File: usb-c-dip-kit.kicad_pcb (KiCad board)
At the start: 2 copper layers, 13.8 x 18.3 mm, 4 parts, among them CN1 USB2.0_C_12pin, CN2 USB_C_DIP_Socket

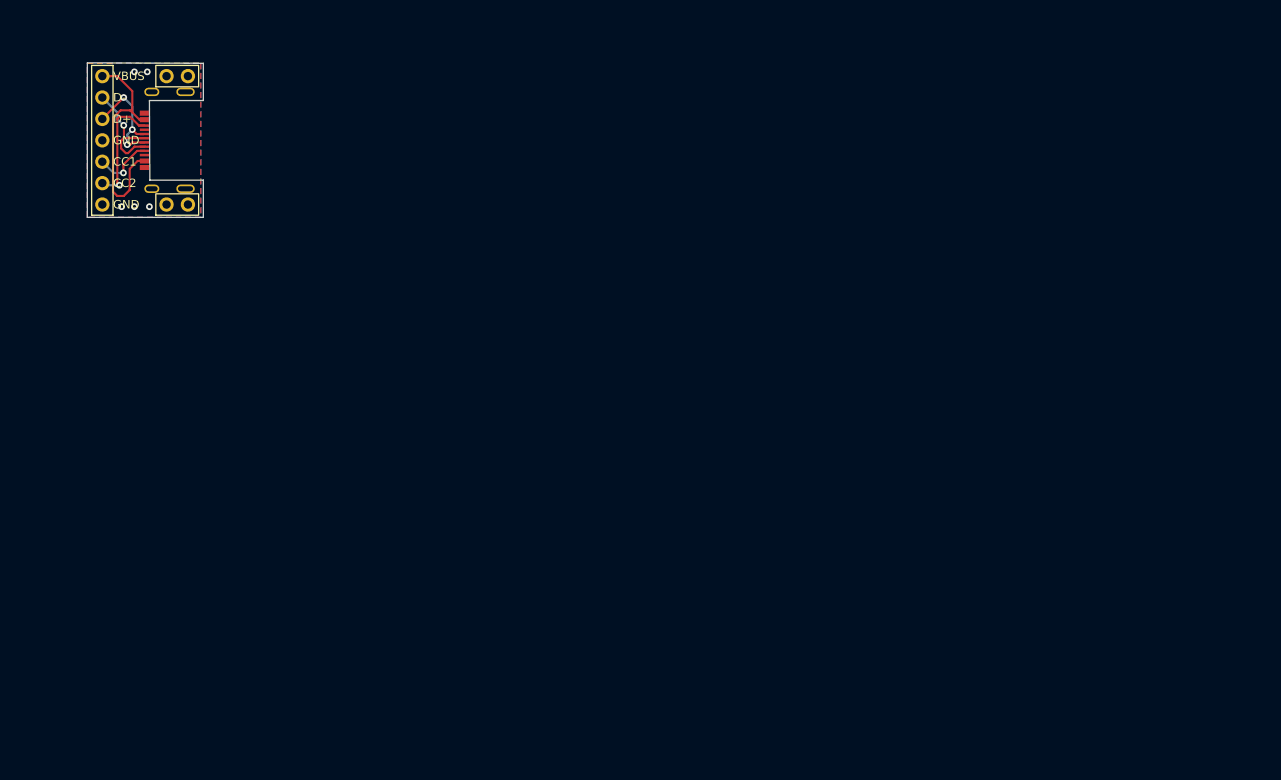
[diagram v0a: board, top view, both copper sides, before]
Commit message: up
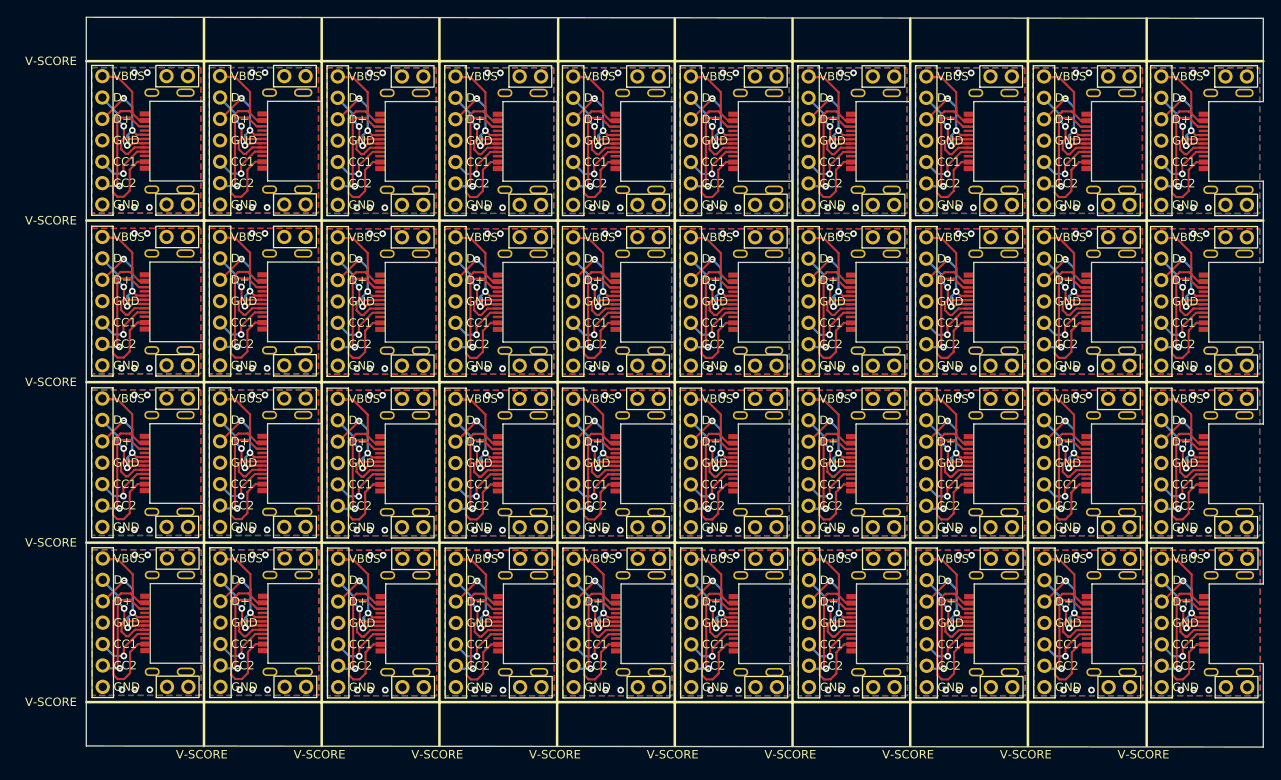
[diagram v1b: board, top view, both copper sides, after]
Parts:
- added CN1: USB2.0_C_12pin, $74th:USB-C-12-Pin-MidMount-ali, F.Cu at (141.0, 95.5)
- added CN1: USB2.0_C_12pin, $74th:USB-C-12-Pin-MidMount-ali, F.Cu at (127.0, 95.5)
- added CN1: USB2.0_C_12pin, $74th:USB-C-12-Pin-MidMount-ali, F.Cu at (113.0, 95.5)
- added CN1: USB2.0_C_12pin, $74th:USB-C-12-Pin-MidMount-ali, F.Cu at (99.0, 76.5)
- added CN1: USB2.0_C_12pin, $74th:USB-C-12-Pin-MidMount-ali, F.Cu at (154.9, 57.3)
- added CN1: USB2.0_C_12pin, $74th:USB-C-12-Pin-MidMount-ali, F.Cu at (113.0, 38.2)
- added CN1: USB2.0_C_12pin, $74th:USB-C-12-Pin-MidMount-ali, F.Cu at (140.9, 38.2)
- added CN1: USB2.0_C_12pin, $74th:USB-C-12-Pin-MidMount-ali, F.Cu at (99.0, 95.5)
- added CN1: USB2.0_C_12pin, $74th:USB-C-12-Pin-MidMount-ali, F.Cu at (99.0, 57.3)
- added CN1: USB2.0_C_12pin, $74th:USB-C-12-Pin-MidMount-ali, F.Cu at (168.8, 95.5)
- added CN1: USB2.0_C_12pin, $74th:USB-C-12-Pin-MidMount-ali, F.Cu at (57.1, 57.3)
- added CN1: USB2.0_C_12pin, $74th:USB-C-12-Pin-MidMount-ali, F.Cu at (71.1, 38.2)
- added CN1: USB2.0_C_12pin, $74th:USB-C-12-Pin-MidMount-ali, F.Cu at (113.0, 57.3)
- added CN1: USB2.0_C_12pin, $74th:USB-C-12-Pin-MidMount-ali, F.Cu at (126.9, 76.5)
- added CN1: USB2.0_C_12pin, $74th:USB-C-12-Pin-MidMount-ali, F.Cu at (71.1, 76.5)
- added CN1: USB2.0_C_12pin, $74th:USB-C-12-Pin-MidMount-ali, F.Cu at (154.9, 76.5)
- added CN1: USB2.0_C_12pin, $74th:USB-C-12-Pin-MidMount-ali, F.Cu at (57.1, 38.2)
- added CN1: USB2.0_C_12pin, $74th:USB-C-12-Pin-MidMount-ali, F.Cu at (168.8, 38.2)
- added CN1: USB2.0_C_12pin, $74th:USB-C-12-Pin-MidMount-ali, F.Cu at (85.0, 57.3)
- added CN1: USB2.0_C_12pin, $74th:USB-C-12-Pin-MidMount-ali, F.Cu at (126.9, 57.3)
- added CN1: USB2.0_C_12pin, $74th:USB-C-12-Pin-MidMount-ali, F.Cu at (168.8, 76.5)
- added CN1: USB2.0_C_12pin, $74th:USB-C-12-Pin-MidMount-ali, F.Cu at (57.1, 95.4)
- added CN1: USB2.0_C_12pin, $74th:USB-C-12-Pin-MidMount-ali, F.Cu at (140.9, 57.3)
- added CN1: USB2.0_C_12pin, $74th:USB-C-12-Pin-MidMount-ali, F.Cu at (43.1, 57.3)
- added CN1: USB2.0_C_12pin, $74th:USB-C-12-Pin-MidMount-ali, F.Cu at (43.2, 95.4)
- added CN1: USB2.0_C_12pin, $74th:USB-C-12-Pin-MidMount-ali, F.Cu at (57.1, 76.5)
- added CN1: USB2.0_C_12pin, $74th:USB-C-12-Pin-MidMount-ali, F.Cu at (85.0, 76.5)
- added CN1: USB2.0_C_12pin, $74th:USB-C-12-Pin-MidMount-ali, F.Cu at (43.1, 76.5)
- added CN1: USB2.0_C_12pin, $74th:USB-C-12-Pin-MidMount-ali, F.Cu at (99.0, 38.2)
- added CN1: USB2.0_C_12pin, $74th:USB-C-12-Pin-MidMount-ali, F.Cu at (154.9, 38.2)
- added CN1: USB2.0_C_12pin, $74th:USB-C-12-Pin-MidMount-ali, F.Cu at (126.9, 38.2)
- added CN1: USB2.0_C_12pin, $74th:USB-C-12-Pin-MidMount-ali, F.Cu at (113.0, 76.5)
- added CN1: USB2.0_C_12pin, $74th:USB-C-12-Pin-MidMount-ali, F.Cu at (140.9, 76.5)
- added CN1: USB2.0_C_12pin, $74th:USB-C-12-Pin-MidMount-ali, F.Cu at (85.0, 38.2)
- added CN1: USB2.0_C_12pin, $74th:USB-C-12-Pin-MidMount-ali, F.Cu at (85.1, 95.5)
- added CN1: USB2.0_C_12pin, $74th:USB-C-12-Pin-MidMount-ali, F.Cu at (71.1, 95.5)
- added CN1: USB2.0_C_12pin, $74th:USB-C-12-Pin-MidMount-ali, F.Cu at (154.9, 95.5)
- added CN1: USB2.0_C_12pin, $74th:USB-C-12-Pin-MidMount-ali, F.Cu at (168.8, 57.3)
- added CN1: USB2.0_C_12pin, $74th:USB-C-12-Pin-MidMount-ali, F.Cu at (71.1, 57.3)
- added CN2: USB_C_DIP_Socket, $usb-type-c-kit:USB2.0-TYPE-C, F.Cu at (135.9, 57.2)
- added CN2: USB_C_DIP_Socket, $usb-type-c-kit:USB2.0-TYPE-C, F.Cu at (52.1, 38.1)
- added CN2: USB_C_DIP_Socket, $usb-type-c-kit:USB2.0-TYPE-C, F.Cu at (163.8, 57.2)
- added CN2: USB_C_DIP_Socket, $usb-type-c-kit:USB2.0-TYPE-C, F.Cu at (108.0, 76.4)
- added CN2: USB_C_DIP_Socket, $usb-type-c-kit:USB2.0-TYPE-C, F.Cu at (163.8, 38.1)
- added CN2: USB_C_DIP_Socket, $usb-type-c-kit:USB2.0-TYPE-C, F.Cu at (80.1, 95.4)
- added CN2: USB_C_DIP_Socket, $usb-type-c-kit:USB2.0-TYPE-C, F.Cu at (121.9, 57.2)
- added CN2: USB_C_DIP_Socket, $usb-type-c-kit:USB2.0-TYPE-C, F.Cu at (108.0, 95.4)
- added CN2: USB_C_DIP_Socket, $usb-type-c-kit:USB2.0-TYPE-C, F.Cu at (108.0, 57.2)
- added CN2: USB_C_DIP_Socket, $usb-type-c-kit:USB2.0-TYPE-C, F.Cu at (52.1, 95.3)
- added CN2: USB_C_DIP_Socket, $usb-type-c-kit:USB2.0-TYPE-C, F.Cu at (149.9, 57.2)
- added CN2: USB_C_DIP_Socket, $usb-type-c-kit:USB2.0-TYPE-C, F.Cu at (94.0, 38.1)
- added CN2: USB_C_DIP_Socket, $usb-type-c-kit:USB2.0-TYPE-C, F.Cu at (80.0, 57.2)
- added CN2: USB_C_DIP_Socket, $usb-type-c-kit:USB2.0-TYPE-C, F.Cu at (38.1, 76.4)
- added CN2: USB_C_DIP_Socket, $usb-type-c-kit:USB2.0-TYPE-C, F.Cu at (66.0, 57.2)
- added CN2: USB_C_DIP_Socket, $usb-type-c-kit:USB2.0-TYPE-C, F.Cu at (163.8, 95.4)
- added CN2: USB_C_DIP_Socket, $usb-type-c-kit:USB2.0-TYPE-C, F.Cu at (80.0, 38.1)
- added CN2: USB_C_DIP_Socket, $usb-type-c-kit:USB2.0-TYPE-C, F.Cu at (121.9, 38.1)
- added CN2: USB_C_DIP_Socket, $usb-type-c-kit:USB2.0-TYPE-C, F.Cu at (66.1, 95.4)
- added CN2: USB_C_DIP_Socket, $usb-type-c-kit:USB2.0-TYPE-C, F.Cu at (52.1, 57.2)
- added CN2: USB_C_DIP_Socket, $usb-type-c-kit:USB2.0-TYPE-C, F.Cu at (121.9, 76.4)
- added CN2: USB_C_DIP_Socket, $usb-type-c-kit:USB2.0-TYPE-C, F.Cu at (135.9, 38.1)
- added CN2: USB_C_DIP_Socket, $usb-type-c-kit:USB2.0-TYPE-C, F.Cu at (66.0, 76.4)
- added CN2: USB_C_DIP_Socket, $usb-type-c-kit:USB2.0-TYPE-C, F.Cu at (149.9, 95.4)
- added CN2: USB_C_DIP_Socket, $usb-type-c-kit:USB2.0-TYPE-C, F.Cu at (94.0, 95.4)
- added CN2: USB_C_DIP_Socket, $usb-type-c-kit:USB2.0-TYPE-C, F.Cu at (122.0, 95.4)
- added CN2: USB_C_DIP_Socket, $usb-type-c-kit:USB2.0-TYPE-C, F.Cu at (38.1, 57.2)
- added CN2: USB_C_DIP_Socket, $usb-type-c-kit:USB2.0-TYPE-C, F.Cu at (149.9, 38.1)
- added CN2: USB_C_DIP_Socket, $usb-type-c-kit:USB2.0-TYPE-C, F.Cu at (80.0, 76.4)
- added CN2: USB_C_DIP_Socket, $usb-type-c-kit:USB2.0-TYPE-C, F.Cu at (94.0, 57.2)
- added CN2: USB_C_DIP_Socket, $usb-type-c-kit:USB2.0-TYPE-C, F.Cu at (38.2, 95.3)
- added CN2: USB_C_DIP_Socket, $usb-type-c-kit:USB2.0-TYPE-C, F.Cu at (108.0, 38.1)
- added CN2: USB_C_DIP_Socket, $usb-type-c-kit:USB2.0-TYPE-C, F.Cu at (149.9, 76.4)
- added CN2: USB_C_DIP_Socket, $usb-type-c-kit:USB2.0-TYPE-C, F.Cu at (66.0, 38.1)
- added CN2: USB_C_DIP_Socket, $usb-type-c-kit:USB2.0-TYPE-C, F.Cu at (163.8, 76.4)
- added CN2: USB_C_DIP_Socket, $usb-type-c-kit:USB2.0-TYPE-C, F.Cu at (52.1, 76.4)
- added CN2: USB_C_DIP_Socket, $usb-type-c-kit:USB2.0-TYPE-C, F.Cu at (135.9, 76.4)
- added CN2: USB_C_DIP_Socket, $usb-type-c-kit:USB2.0-TYPE-C, F.Cu at (135.9, 95.4)
- added CN2: USB_C_DIP_Socket, $usb-type-c-kit:USB2.0-TYPE-C, F.Cu at (94.0, 76.4)
- added REF**: Mount_2Pin, $74th:Mount_2Pin, F.Cu at (116.9, 103.0)
- added REF**: Mount_2Pin, $74th:Mount_2Pin, F.Cu at (116.8, 45.8)
- added REF**: Mount_2Pin, $74th:Mount_2Pin, F.Cu at (144.8, 103.0)
- added REF**: Mount_2Pin, $74th:Mount_2Pin, F.Cu at (144.8, 45.8)
- added REF**: Mount_2Pin, $74th:Mount_2Pin, F.Cu at (144.8, 64.8)
- added REF**: Mount_2Pin, $74th:Mount_2Pin, F.Cu at (144.8, 84.0)
- added REF**: Mount_2Pin, $74th:Mount_2Pin, F.Cu at (130.8, 64.8)
- added REF**: Mount_2Pin, $74th:Mount_2Pin, F.Cu at (88.9, 49.6)
- added REF**: Mount_2Pin, $74th:Mount_2Pin, F.Cu at (75.0, 87.8)
- added REF**: Mount_2Pin, $74th:Mount_2Pin, F.Cu at (102.9, 30.5)
- added REF**: Mount_2Pin, $74th:Mount_2Pin, F.Cu at (158.8, 49.6)
- added REF**: Mount_2Pin, $74th:Mount_2Pin, F.Cu at (144.8, 30.5)
- added REF**: Mount_2Pin, $74th:Mount_2Pin, F.Cu at (89.0, 87.8)
- added REF**: Mount_2Pin, $74th:Mount_2Pin, F.Cu at (116.8, 64.8)
- added REF**: Mount_2Pin, $74th:Mount_2Pin, F.Cu at (130.8, 30.5)
- added REF**: Mount_2Pin, $74th:Mount_2Pin, F.Cu at (88.9, 30.5)
- added REF**: Mount_2Pin, $74th:Mount_2Pin, F.Cu at (74.9, 64.8)
- added REF**: Mount_2Pin, $74th:Mount_2Pin, F.Cu at (116.8, 68.8)
- added REF**: Mount_2Pin, $74th:Mount_2Pin, F.Cu at (88.9, 64.8)
- added REF**: Mount_2Pin, $74th:Mount_2Pin, F.Cu at (88.9, 84.0)
- added REF**: Mount_2Pin, $74th:Mount_2Pin, F.Cu at (144.8, 49.6)
- added REF**: Mount_2Pin, $74th:Mount_2Pin, F.Cu at (158.8, 45.8)
- added REF**: Mount_2Pin, $74th:Mount_2Pin, F.Cu at (102.9, 45.8)
- added REF**: Mount_2Pin, $74th:Mount_2Pin, F.Cu at (88.9, 45.8)
- added REF**: Mount_2Pin, $74th:Mount_2Pin, F.Cu at (102.9, 84.0)
- added REF**: Mount_2Pin, $74th:Mount_2Pin, F.Cu at (116.9, 87.8)
- added REF**: Mount_2Pin, $74th:Mount_2Pin, F.Cu at (158.8, 84.0)
- added REF**: Mount_2Pin, $74th:Mount_2Pin, F.Cu at (172.7, 45.8)
- added REF**: Mount_2Pin, $74th:Mount_2Pin, F.Cu at (74.9, 45.8)
- added REF**: Mount_2Pin, $74th:Mount_2Pin, F.Cu at (130.8, 68.8)
- added REF**: Mount_2Pin, $74th:Mount_2Pin, F.Cu at (61.0, 49.6)
- added REF**: Mount_2Pin, $74th:Mount_2Pin, F.Cu at (172.7, 84.0)
- added REF**: Mount_2Pin, $74th:Mount_2Pin, F.Cu at (61.0, 64.8)
- added REF**: Mount_2Pin, $74th:Mount_2Pin, F.Cu at (130.9, 87.8)
- added REF**: Mount_2Pin, $74th:Mount_2Pin, F.Cu at (47.0, 84.0)
- added REF**: Mount_2Pin, $74th:Mount_2Pin, F.Cu at (116.8, 49.6)
- added REF**: Mount_2Pin, $74th:Mount_2Pin, F.Cu at (89.0, 103.0)
- added REF**: Mount_2Pin, $74th:Mount_2Pin, F.Cu at (158.8, 64.8)
- added REF**: Mount_2Pin, $74th:Mount_2Pin, F.Cu at (47.0, 49.6)
- added REF**: Mount_2Pin, $74th:Mount_2Pin, F.Cu at (74.9, 68.8)
- added REF**: Mount_2Pin, $74th:Mount_2Pin, F.Cu at (61.0, 68.7)
- added REF**: Mount_2Pin, $74th:Mount_2Pin, F.Cu at (61.0, 45.7)
- added REF**: Mount_2Pin, $74th:Mount_2Pin, F.Cu at (172.7, 30.5)
- added REF**: Mount_2Pin, $74th:Mount_2Pin, F.Cu at (172.7, 68.8)
- added REF**: Mount_2Pin, $74th:Mount_2Pin, F.Cu at (102.9, 49.6)
- added REF**: Mount_2Pin, $74th:Mount_2Pin, F.Cu at (158.8, 68.8)
- added REF**: Mount_2Pin, $74th:Mount_2Pin, F.Cu at (47.0, 68.7)
- added REF**: Mount_2Pin, $74th:Mount_2Pin, F.Cu at (172.7, 64.8)
- added REF**: Mount_2Pin, $74th:Mount_2Pin, F.Cu at (130.9, 103.0)
- added REF**: Mount_2Pin, $74th:Mount_2Pin, F.Cu at (74.9, 84.0)
- added REF**: Mount_2Pin, $74th:Mount_2Pin, F.Cu at (74.9, 30.5)
- added REF**: Mount_2Pin, $74th:Mount_2Pin, F.Cu at (61.0, 103.0)
- added REF**: Mount_2Pin, $74th:Mount_2Pin, F.Cu at (102.9, 103.0)
- added REF**: Mount_2Pin, $74th:Mount_2Pin, F.Cu at (61.0, 30.5)
- added REF**: Mount_2Pin, $74th:Mount_2Pin, F.Cu at (61.0, 87.7)
- added REF**: Mount_2Pin, $74th:Mount_2Pin, F.Cu at (144.8, 87.8)
- added REF**: Mount_2Pin, $74th:Mount_2Pin, F.Cu at (172.7, 87.8)
- added REF**: Mount_2Pin, $74th:Mount_2Pin, F.Cu at (158.8, 30.5)
- added REF**: Mount_2Pin, $74th:Mount_2Pin, F.Cu at (102.9, 64.8)
- added REF**: Mount_2Pin, $74th:Mount_2Pin, F.Cu at (47.0, 87.7)
- added REF**: Mount_2Pin, $74th:Mount_2Pin, F.Cu at (130.8, 84.0)
- added REF**: Mount_2Pin, $74th:Mount_2Pin, F.Cu at (116.8, 30.5)
- added REF**: Mount_2Pin, $74th:Mount_2Pin, F.Cu at (144.8, 68.8)
- added REF**: Mount_2Pin, $74th:Mount_2Pin, F.Cu at (75.0, 103.0)
- added REF**: Mount_2Pin, $74th:Mount_2Pin, F.Cu at (61.0, 84.0)
- added REF**: Mount_2Pin, $74th:Mount_2Pin, F.Cu at (47.0, 103.0)
- added REF**: Mount_2Pin, $74th:Mount_2Pin, F.Cu at (158.8, 87.8)
- added REF**: Mount_2Pin, $74th:Mount_2Pin, F.Cu at (102.9, 68.8)
- added REF**: Mount_2Pin, $74th:Mount_2Pin, F.Cu at (88.9, 68.8)
- added REF**: Mount_2Pin, $74th:Mount_2Pin, F.Cu at (172.7, 103.0)
- added REF**: Mount_2Pin, $74th:Mount_2Pin, F.Cu at (102.9, 87.8)
- added REF**: Mount_2Pin, $74th:Mount_2Pin, F.Cu at (158.8, 103.0)
- added REF**: Mount_2Pin, $74th:Mount_2Pin, F.Cu at (74.9, 49.6)
- added REF**: Mount_2Pin, $74th:Mount_2Pin, F.Cu at (172.7, 49.6)
- added REF**: Mount_2Pin, $74th:Mount_2Pin, F.Cu at (130.8, 49.6)
- added REF**: Mount_2Pin, $74th:Mount_2Pin, F.Cu at (116.8, 84.0)
- added REF**: Mount_2Pin, $74th:Mount_2Pin, F.Cu at (47.0, 64.8)
- added REF**: Mount_2Pin, $74th:Mount_2Pin, F.Cu at (130.8, 45.8)
- moved CN1 0.09 mm to (43.1, 38.2)
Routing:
- net Net-(CN1-Pad11): track 28.3 -> 1132.9 mm
- net Net-(CN1-Pad10): track 13.9 -> 555.5 mm, vias 1 -> 40
- net Net-(CN1-Pad6): track 13.7 -> 547.9 mm, vias 3 -> 120
- net Net-(CN1-Pad5): track 13.5 -> 539.6 mm, vias 1 -> 40
- net Net-(CN1-Pad4): track 7.21 -> 288.5 mm, vias 1 -> 40
- net Net-(CN1-Pad1): vias 5 -> 200
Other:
- board size 13.8 x 18.3 mm -> 139.7 x 86.6 mm
- board text added: "V-SCORE"

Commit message: up
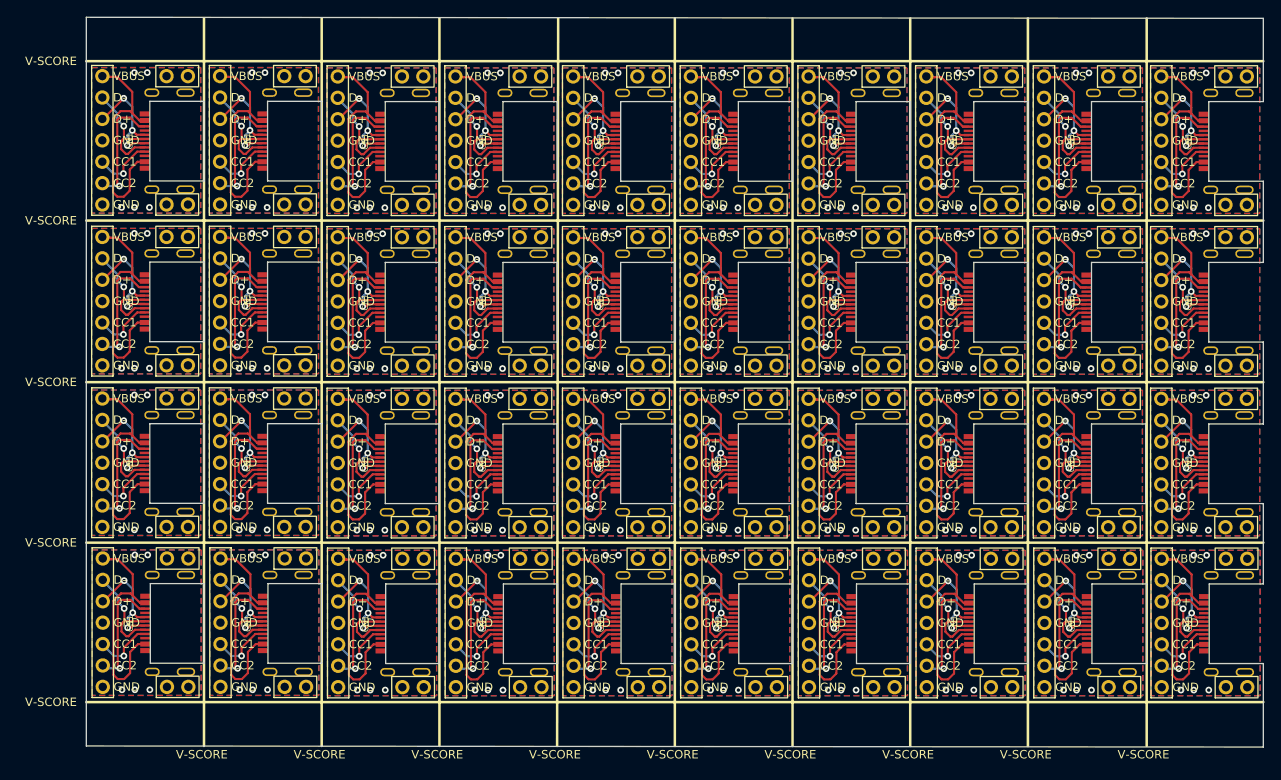
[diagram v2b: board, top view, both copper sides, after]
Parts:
- CN1 (x40): footprint $74th:USB-C-12-Pin-MidMount-ali -> $usb-type-c-kit:USB-C-12-Pin-MidMount-ali

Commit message: v2
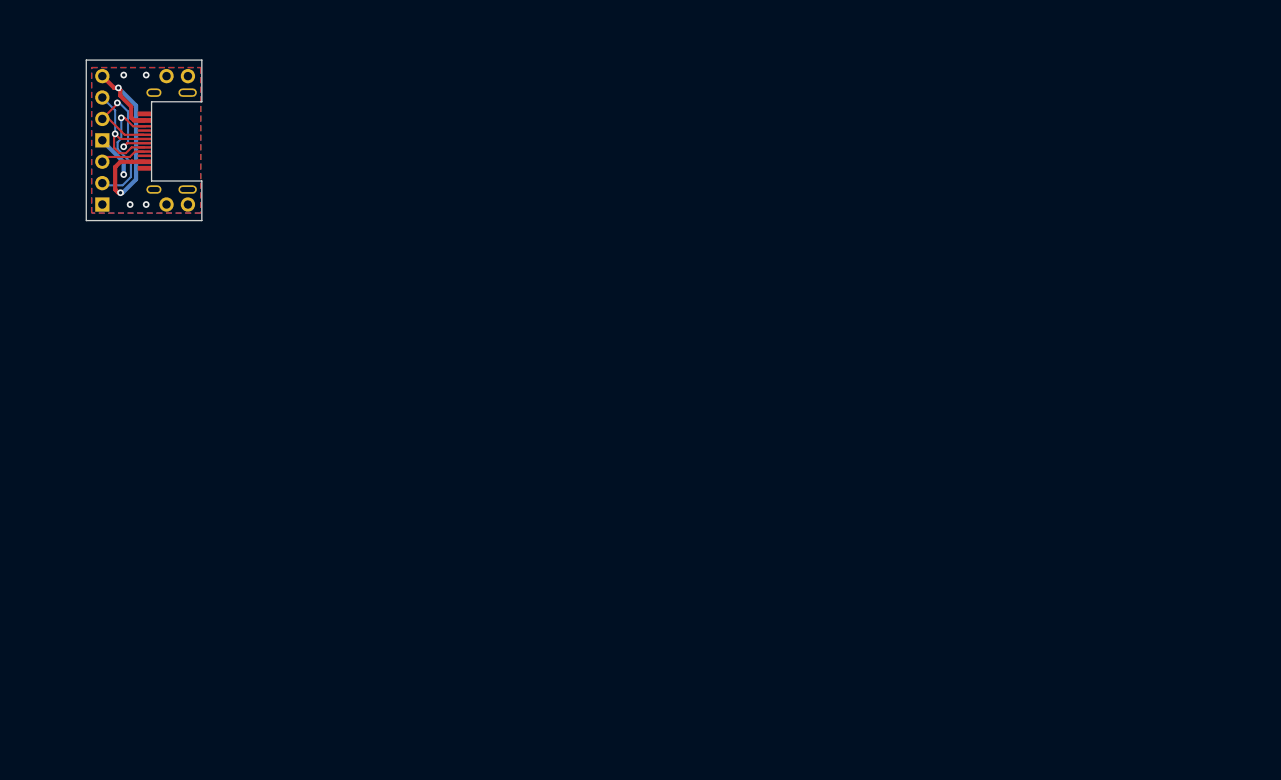
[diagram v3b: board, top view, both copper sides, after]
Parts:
- removed the CN1 at (141.0, 95.5)
- removed the CN1 at (127.0, 95.5)
- removed the CN1 at (113.0, 95.5)
- removed the CN1 at (99.0, 76.5)
- removed the CN1 at (154.9, 57.3)
- removed the CN1 at (113.0, 38.2)
- removed the CN1 at (140.9, 38.2)
- removed the CN1 at (99.0, 95.5)
- removed the CN1 at (99.0, 57.3)
- removed the CN1 at (168.8, 95.5)
- removed the CN1 at (57.1, 57.3)
- removed the CN1 at (71.1, 38.2)
- removed the CN1 at (113.0, 57.3)
- removed the CN1 at (126.9, 76.5)
- removed the CN1 at (71.1, 76.5)
- removed the CN1 at (154.9, 76.5)
- removed the CN1 at (57.1, 38.2)
- removed the CN1 at (168.8, 38.2)
- removed the CN1 at (85.0, 57.3)
- removed the CN1 at (126.9, 57.3)
- removed the CN1 at (168.8, 76.5)
- removed the CN1 at (57.1, 95.4)
- removed the CN1 at (140.9, 57.3)
- removed the CN1 at (43.1, 57.3)
- removed the CN1 at (43.2, 95.4)
- removed the CN1 at (57.1, 76.5)
- removed the CN1 at (85.0, 76.5)
- removed the CN1 at (43.1, 76.5)
- removed the CN1 at (99.0, 38.2)
- removed the CN1 at (154.9, 38.2)
- removed the CN1 at (126.9, 38.2)
- removed the CN1 at (113.0, 76.5)
- removed the CN1 at (140.9, 76.5)
- removed the CN1 at (85.0, 38.2)
- removed the CN1 at (85.1, 95.5)
- removed the CN1 at (71.1, 95.5)
- removed the CN1 at (154.9, 95.5)
- removed the CN1 at (168.8, 57.3)
- removed the CN1 at (71.1, 57.3)
- removed the CN2 at (135.9, 57.2)
- removed the CN2 at (52.1, 38.1)
- removed the CN2 at (163.8, 57.2)
- removed the CN2 at (108.0, 76.4)
- removed the CN2 at (163.8, 38.1)
- removed the CN2 at (80.1, 95.4)
- removed the CN2 at (121.9, 57.2)
- removed the CN2 at (108.0, 95.4)
- removed the CN2 at (108.0, 57.2)
- removed the CN2 at (52.1, 95.3)
- removed the CN2 at (149.9, 57.2)
- removed the CN2 at (94.0, 38.1)
- removed the CN2 at (80.0, 57.2)
- removed the CN2 at (38.1, 76.4)
- removed the CN2 at (66.0, 57.2)
- removed the CN2 at (163.8, 95.4)
- removed the CN2 at (80.0, 38.1)
- removed the CN2 at (121.9, 38.1)
- removed the CN2 at (66.1, 95.4)
- removed the CN2 at (52.1, 57.2)
- removed the CN2 at (121.9, 76.4)
- removed the CN2 at (135.9, 38.1)
- removed the CN2 at (66.0, 76.4)
- removed the CN2 at (149.9, 95.4)
- removed the CN2 at (94.0, 95.4)
- removed the CN2 at (122.0, 95.4)
- removed the CN2 at (38.1, 57.2)
- removed the CN2 at (149.9, 38.1)
- removed the CN2 at (80.0, 76.4)
- removed the CN2 at (94.0, 57.2)
- removed the CN2 at (38.2, 95.3)
- removed the CN2 at (108.0, 38.1)
- removed the CN2 at (149.9, 76.4)
- removed the CN2 at (66.0, 38.1)
- removed the CN2 at (163.8, 76.4)
- removed the CN2 at (52.1, 76.4)
- removed the CN2 at (135.9, 76.4)
- removed the CN2 at (135.9, 95.4)
- removed the CN2 at (94.0, 76.4)
- removed the REF** at (116.9, 103.0)
- removed the REF** at (116.8, 45.8)
- removed the REF** at (144.8, 103.0)
- removed the REF** at (144.8, 45.8)
- removed the REF** at (144.8, 64.8)
- removed the REF** at (144.8, 84.0)
- removed the REF** at (130.8, 64.8)
- removed the REF** at (88.9, 49.6)
- removed the REF** at (75.0, 87.8)
- removed the REF** at (102.9, 30.5)
- removed the REF** at (158.8, 49.6)
- removed the REF** at (144.8, 30.5)
- removed the REF** at (89.0, 87.8)
- removed the REF** at (116.8, 64.8)
- removed the REF** at (130.8, 30.5)
- removed the REF** at (88.9, 30.5)
- removed the REF** at (74.9, 64.8)
- removed the REF** at (116.8, 68.8)
- removed the REF** at (88.9, 64.8)
- removed the REF** at (88.9, 84.0)
- removed the REF** at (144.8, 49.6)
- removed the REF** at (158.8, 45.8)
- removed the REF** at (102.9, 45.8)
- removed the REF** at (88.9, 45.8)
- removed the REF** at (102.9, 84.0)
- removed the REF** at (116.9, 87.8)
- removed the REF** at (158.8, 84.0)
- removed the REF** at (172.7, 45.8)
- removed the REF** at (74.9, 45.8)
- removed the REF** at (130.8, 68.8)
- removed the REF** at (61.0, 49.6)
- removed the REF** at (172.7, 84.0)
- removed the REF** at (61.0, 64.8)
- removed the REF** at (130.9, 87.8)
- removed the REF** at (47.0, 84.0)
- removed the REF** at (116.8, 49.6)
- removed the REF** at (89.0, 103.0)
- removed the REF** at (158.8, 64.8)
- removed the REF** at (47.0, 49.6)
- removed the REF** at (74.9, 68.8)
- removed the REF** at (61.0, 68.7)
- removed the REF** at (61.0, 45.7)
- removed the REF** at (172.7, 30.5)
- removed the REF** at (172.7, 68.8)
- removed the REF** at (102.9, 49.6)
- removed the REF** at (158.8, 68.8)
- removed the REF** at (47.0, 68.7)
- removed the REF** at (172.7, 64.8)
- removed the REF** at (130.9, 103.0)
- removed the REF** at (74.9, 84.0)
- removed the REF** at (74.9, 30.5)
- removed the REF** at (61.0, 103.0)
- removed the REF** at (102.9, 103.0)
- removed the REF** at (61.0, 30.5)
- removed the REF** at (61.0, 87.7)
- removed the REF** at (144.8, 87.8)
- removed the REF** at (172.7, 87.8)
- removed the REF** at (158.8, 30.5)
- removed the REF** at (102.9, 64.8)
- removed the REF** at (47.0, 87.7)
- removed the REF** at (130.8, 84.0)
- removed the REF** at (116.8, 30.5)
- removed the REF** at (144.8, 68.8)
- removed the REF** at (75.0, 103.0)
- removed the REF** at (61.0, 84.0)
- removed the REF** at (47.0, 103.0)
- removed the REF** at (158.8, 87.8)
- removed the REF** at (102.9, 68.8)
- removed the REF** at (88.9, 68.8)
- removed the REF** at (172.7, 103.0)
- removed the REF** at (102.9, 87.8)
- removed the REF** at (158.8, 103.0)
- removed the REF** at (74.9, 49.6)
- removed the REF** at (172.7, 49.6)
- removed the REF** at (130.8, 49.6)
- removed the REF** at (116.8, 84.0)
- removed the REF** at (47.0, 64.8)
- removed the REF** at (130.8, 45.8)
- CN1: footprint $usb-type-c-kit:USB-C-12-Pin-MidMount-ali -> $74th:USB-C-12-Pin-MidMount-ali-v2
- CN2: footprint $usb-type-c-kit:USB2.0-TYPE-C -> $usb-type-c-kit:USB2.0-TYPE-C-NOSILK
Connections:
- net Net-(CN1-Pad1) renamed GND
- net Net-(CN1-Pad11) renamed +5V
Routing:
- net +5V: track 1132.9 -> 29.8 mm, vias 0 -> 2
- net Net-(CN1-Pad10): track 555.5 -> 15.0 mm, vias 40 -> 1
- net Net-(CN1-Pad6): track 547.9 -> 17.2 mm, vias 120 -> 2
- net Net-(CN1-Pad5): track 539.6 -> 14.6 mm, vias 40 -> 1
- net Net-(CN1-Pad4): track 288.5 -> 5.51 mm, vias 40 -> 0
- net GND: track 0.00 -> 5.12 mm, vias 200 -> 5
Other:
- board size 139.7 x 86.6 mm -> 13.7 x 19.1 mm
- board text removed: "V-SCORE"
